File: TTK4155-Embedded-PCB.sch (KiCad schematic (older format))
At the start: 45 parts, among them J1 AVR-JTAG-10, J2 DB9_Female, J3 Conn_01x10_Male, J4 Conn_01x04_Male, J5 Screw_Terminal_01x02, J6 Screw_Terminal_01x02, J7 Conn_01x04_Male, J8 BannanaJack, SW1 SW_Push, U1 L7805, U2 ATmega162-16PU, U3 IDT7164S, U4 GAL16V8, U5 SN74ALS573CN, U6 MCP2515-18PDIP, U7 MCP2551-I-P, U8 MAX233, U9 ADC0844, Y1 4,9152MHz, Y2 16.0MHz

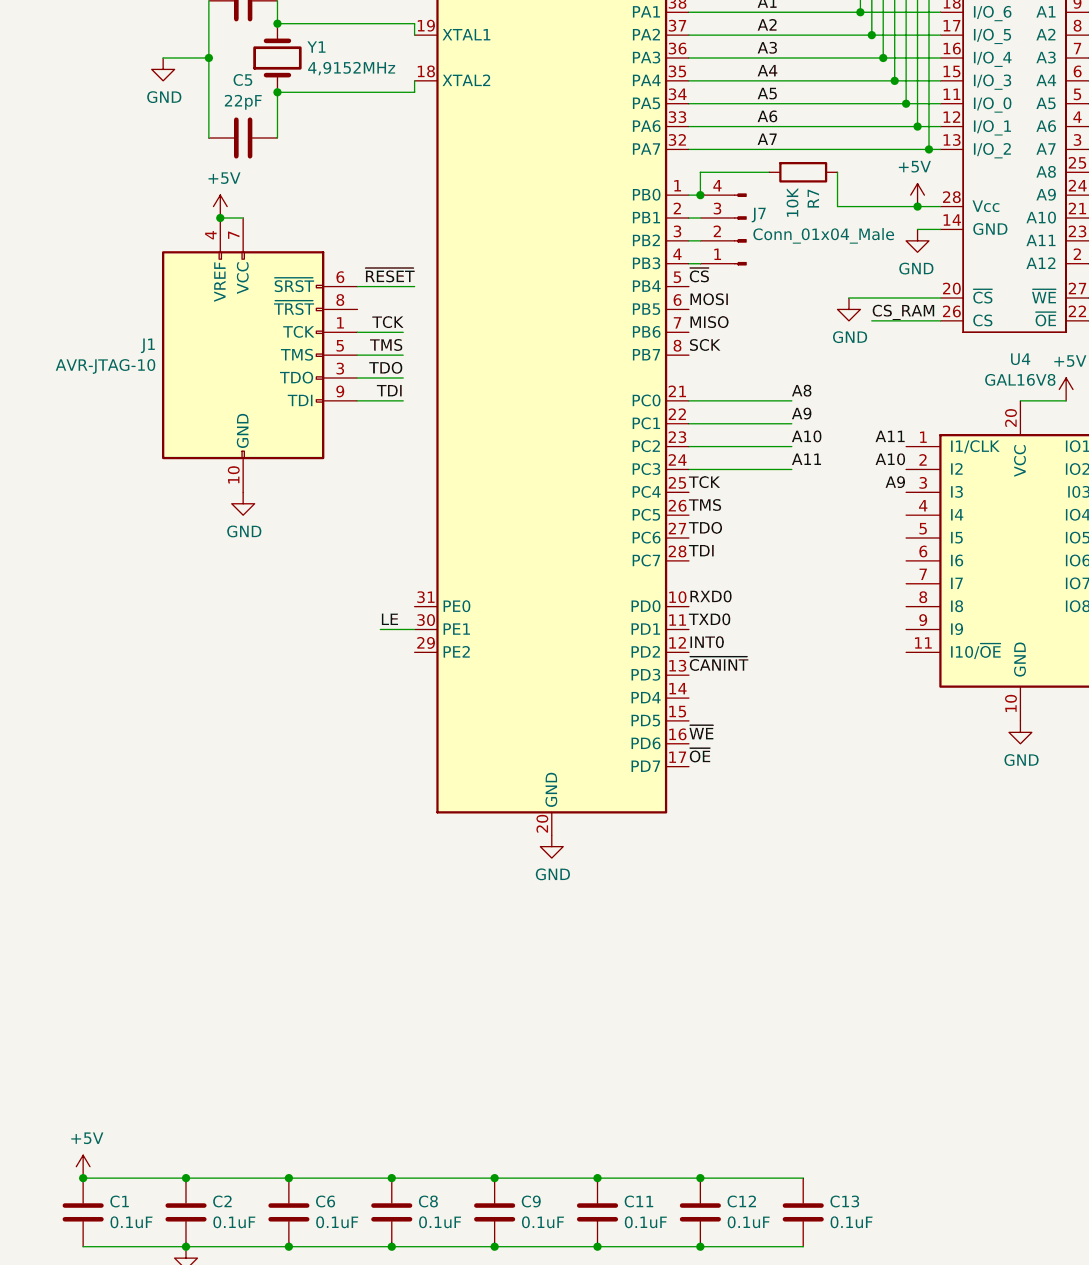
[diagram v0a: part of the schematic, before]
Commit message: Made som esmall changes and send pcb to production
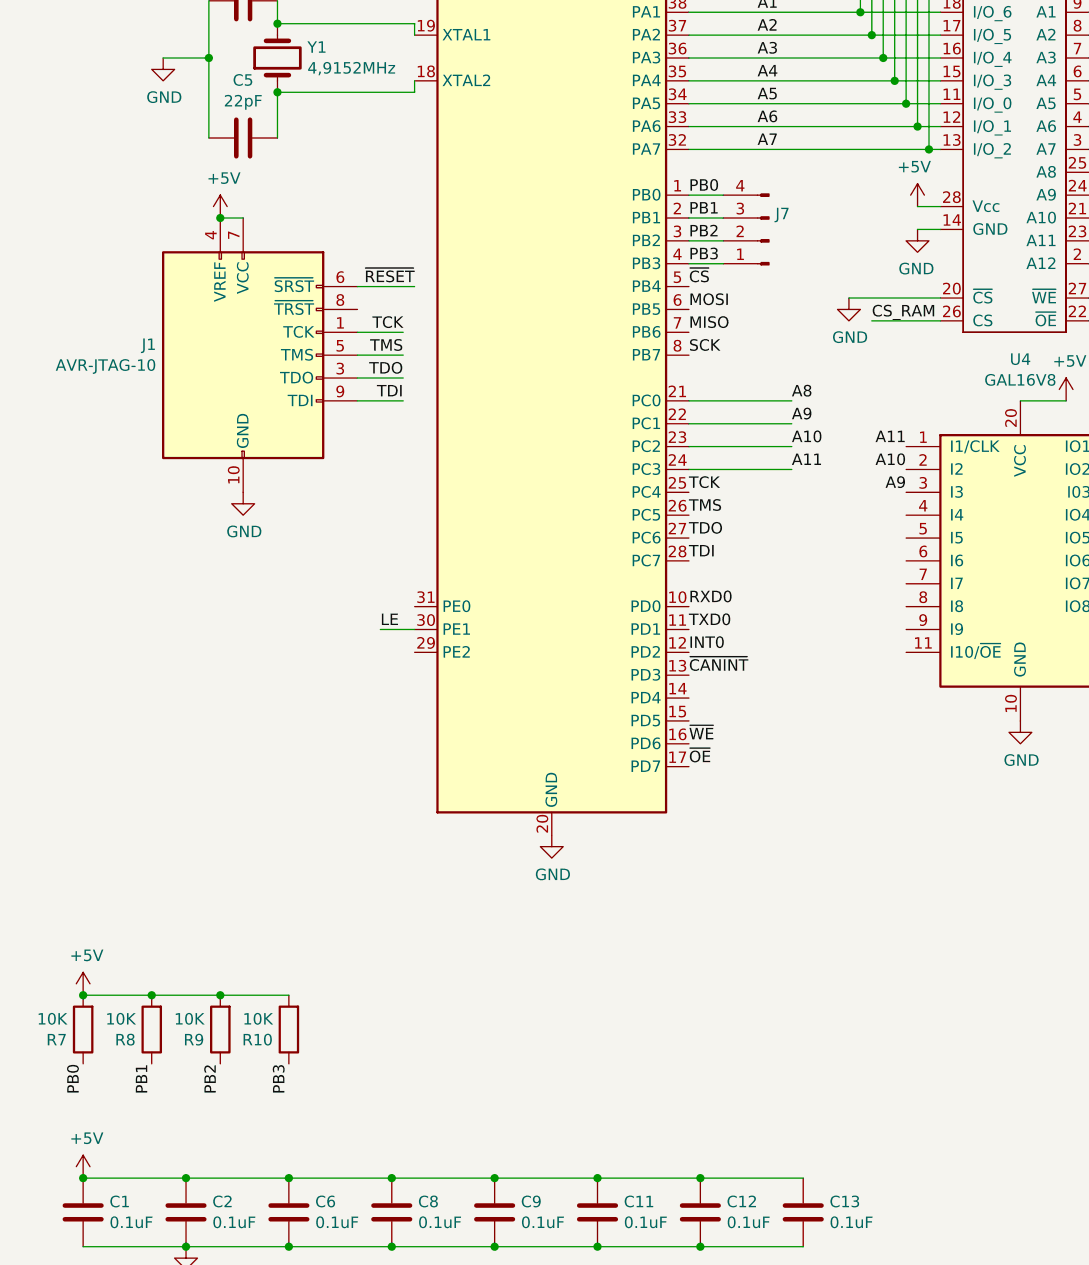
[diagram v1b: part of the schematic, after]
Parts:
- added R10, R8, R9: 10K, Resistor_SMD:R_0805_2012Metric_Pad1.15x1.40mm_HandSolder, symbol Device:R
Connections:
- net +5V: now also R7.2, R10.2, R8.2, R9.2; no longer R7.1
- net PB0: now reaches J7.4 (Pin_4), U2.1 (PB0)
- net PB0: now also R7.1; no longer R7.2
- net PB1: now reaches J7.3 (Pin_3), U2.2 (PB1)
- net PB1: now also R8.1
- net PB2: now reaches J7.2 (Pin_2), U2.3 (PB2)
- net PB2: now also R9.1
- net PB3: now reaches J7.1 (Pin_1), U2.4 (PB3)
- net PB3: now also R10.1
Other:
- moved on the sheet: J7
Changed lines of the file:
@@
 L Connector:Conn_01x04_Male J7
 U 1 1 5DDF74B0
-P 3600 3000
-F 0 "J7" H 3572 2882 50  0000 R CNN
-F 1 "Conn_01x04_Male" H 3572 2973 50  0000 R CNN
-F 2 "Connector_PinHeader_2.54mm:PinHeader_1x04_P2.54mm_Vertical" H 3600 3000 50  0001 C CNN
-F 3 "~" H 3600 3000 50  0001 C CNN
-	1    3600 3000
+P 3700 3000
+F 0 "J7" H 3672 2882 50  0000 R CNN
+F 1 "Conn_01x04_Male" H 3672 2973 50  0001 R CNN
+F 2 "Connector_PinHeader_2.54mm:PinHeader_1x04_P2.54mm_Vertical" H 3700 3000 50  0001 C CNN
+F 3 "~" H 3700 3000 50  0001 C CNN
+	1    3700 3000
 	-1   0    0    1
 $EndComp
@@
 $Comp
 L Device:R R7
-U 1 1 5DF418AD
-P 3850 2700
-F 0 "R7" H 3920 2746 50  0000 L CNN
-F 1 "10K" H 3920 2655 50  0000 L CNN
-F 2 "Resistor_SMD:R_0805_2012Metric_Pad1.15x1.40mm_HandSolder" V 3780 2700 50  0001 C CNN
-F 3 "~" H 3850 2700 50  0001 C CNN
-	1    3850 2700
-	0    1    1    0
+U 1 1 5DB3F4E5
+P 700 6450
+F 0 "R7" H 770 6496 50  0000 L CNN
+F 1 "10K" H 770 6405 50  0000 L CNN
+F 2 "Resistor_SMD:R_0805_2012Metric_Pad1.15x1.40mm_HandSolder" V 630 6450 50  0001 C CNN
+F 3 "~" H 700 6450 50  0001 C CNN
+	1    700  6450
+	-1   0    0    1
+$EndComp
+Text Label 3350 2800 0    50   ~ 0
+PB0
+Text Label 3350 2900 0    50   ~ 0
+PB1
+Text Label 3350 3000 0    50   ~ 0
+PB2
+Text Label 3350 3100 0    50   ~ 0
+PB3
+Wire Wire Line
+	3350 2800 3500 2800
+Wire Wire Line
+	3350 2900 3500 2900
+Wire Wire Line
+	3350 3000 3500 3000
+Wire Wire Line
+	3350 3100 3500 3100
+$Comp
+L Device:R R8
+U 1 1 5DB7ED57
+P 1000 6450
+F 0 "R8" H 1070 6496 50  0000 L CNN
+F 1 "10K" H 1070 6405 50  0000 L CNN
+F 2 "Resistor_SMD:R_0805_2012Metric_Pad1.15x1.40mm_HandSolder" V 930 6450 50  0001 C CNN
+F 3 "~" H 1000 6450 50  0001 C CNN
+	1    1000 6450
+	-1   0    0    1
+$EndComp
+$Comp
+L Device:R R9
+U 1 1 5DB7F993
+P 1300 6450
+F 0 "R9" H 1370 6496 50  0000 L CNN
+F 1 "10K" H 1370 6405 50  0000 L CNN
+F 2 "Resistor_SMD:R_0805_2012Metric_Pad1.15x1.40mm_HandSolder" V 1230 6450 50  0001 C CNN
+F 3 "~" H 1300 6450 50  0001 C CNN
+	1    1300 6450
+	-1   0    0    1
+$EndComp
+$Comp
+L Device:R R10
+U 1 1 5DB7F999
+P 1600 6450
+F 0 "R10" H 1670 6496 50  0000 L CNN
+F 1 "10K" H 1670 6405 50  0000 L CNN
+F 2 "Resistor_SMD:R_0805_2012Metric_Pad1.15x1.40mm_HandSolder" V 1530 6450 50  0001 C CNN
+F 3 "~" H 1600 6450 50  0001 C CNN
+	1    1600 6450
+	-1   0    0    1
+$EndComp
+$Comp
+L power:+5V #PWR0138
+U 1 1 5DB8E098
+P 700 6300
+F 0 "#PWR0138" H 700 6150 50  0001 C CNN
+F 1 "+5V" H 715 6473 50  0000 C CNN
+F 2 "" H 700 6300 50  0001 C CNN
+F 3 "" H 700 6300 50  0001 C CNN
+	1    700  6300
+	1    0    0    -1
 $EndComp
 Wire Wire Line
-	3350 2800 3400 2800
+	1600 6300 1300 6300
+Connection ~ 700  6300
+Connection ~ 1000 6300
 Wire Wire Line
-	3400 2800 3400 2700
+	1000 6300 700  6300
+Connection ~ 1300 6300
 Wire Wire Line
-	3400 2700 3700 2700
-Connection ~ 3400 2800
-Wire Wire Line
-	3350 2900 3400 2900
-Wire Wire Line
-	3350 3000 3400 3000
-Wire Wire Line
-	3350 3100 3400 3100
-Wire Wire Line
-	4000 2700 4000 2850
-Wire Wire Line
-	4000 2850 4350 2850
-Connection ~ 4350 2850
+	1300 6300 1000 6300
+Text Label 700  6600 3    50   ~ 0
+PB0
+Text Label 1000 6600 3    50   ~ 0
+PB1
+Text Label 1300 6600 3    50   ~ 0
+PB2
+Text Label 1600 6600 3    50   ~ 0
+PB3
 $EndSCHEMATC
